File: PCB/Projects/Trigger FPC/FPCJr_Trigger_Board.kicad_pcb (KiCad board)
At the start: 2 copper layers, 56.2 x 14.3 mm, 6 parts, among them J1 Conn_01x04_Pin, J2 Conn_01x04_Pin, U1 HAL4395, U2 HAL4395

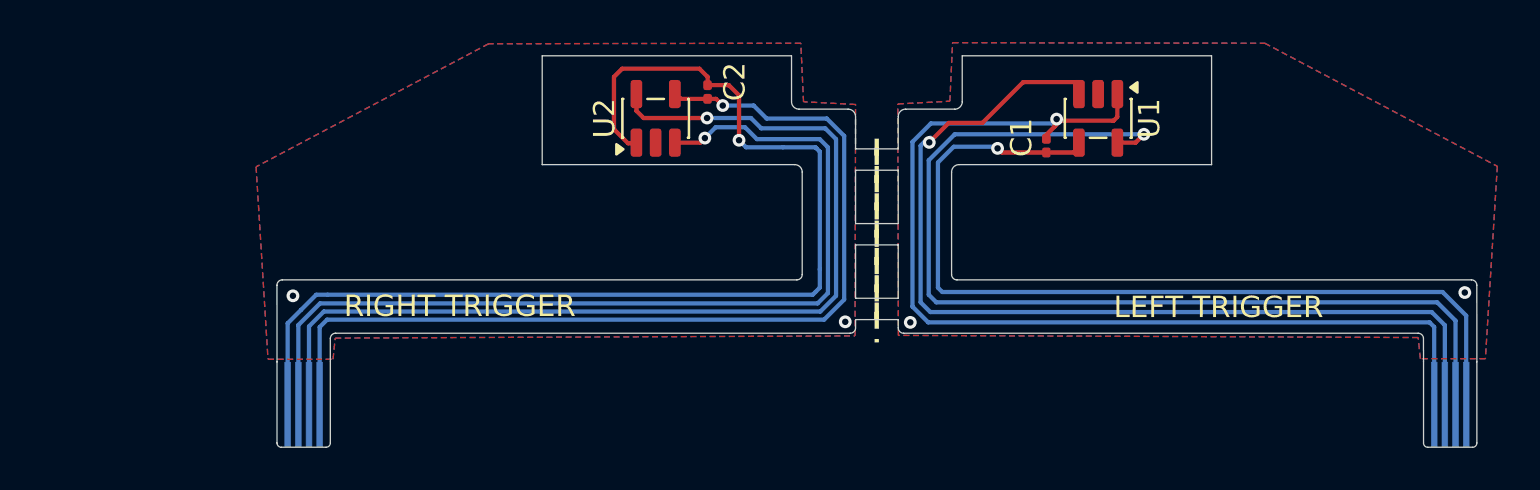
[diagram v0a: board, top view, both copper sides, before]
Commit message: FPC Board Update
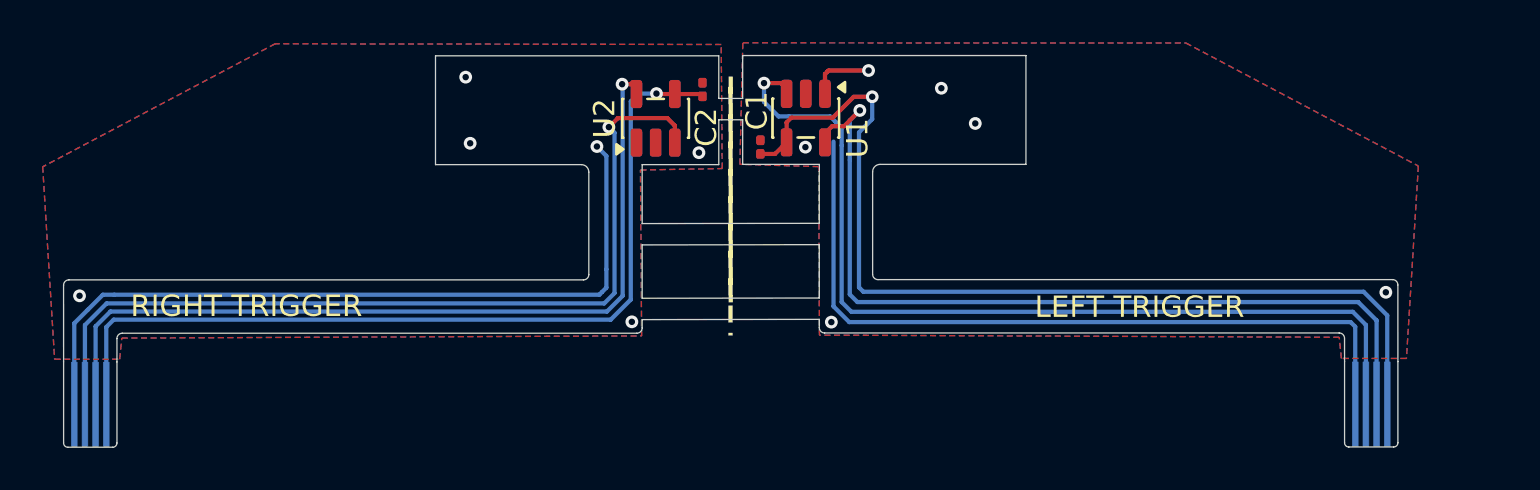
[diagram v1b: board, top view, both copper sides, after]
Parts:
- moved U1 13.7 mm to (250.4, 148.9)
- moved C1 13.4 mm to (248.3, 150.3)
- moved J1 10.0 mm to (216.9, 162.4)
- moved J2 3.70 mm to (276.9, 162.4)
- moved C2 0.26 mm to (245.6, 147.6)
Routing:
- net GND: track 52.5 -> 36.2 mm, vias 3 -> 6
- net GNDL: track 48.7 -> 39.2 mm, vias 3 -> 6
- net TRIGGER_EN_L: track 48.1 -> 40.4 mm
- net TRIGGER_EN_R: track 47.0 -> 40.0 mm
- net +3V3: track 45.1 -> 41.6 mm
- net +3V3L: track 42.7 -> 45.6 mm
- net ADC_1: track 43.9 -> 41.3 mm
- net ADC_0: track 45.1 -> 43.3 mm
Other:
- board size 56.2 x 14.3 mm -> 62.5 x 14.4 mm
